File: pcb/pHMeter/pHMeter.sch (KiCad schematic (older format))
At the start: 75 parts, among them J1 Conn_02x03_Odd_Even, J2 Conn_Coaxial_Power, J3 Conn_Coaxial_Power, J4 Conn_Coaxial_Power, J5 RJ12, J6 RJ12, Q1 BSP75, Q2 BSP75, U1 TLV6004PW, U2 TLV6004PW, X1 MINI-USB-SCHIELD-32005-201

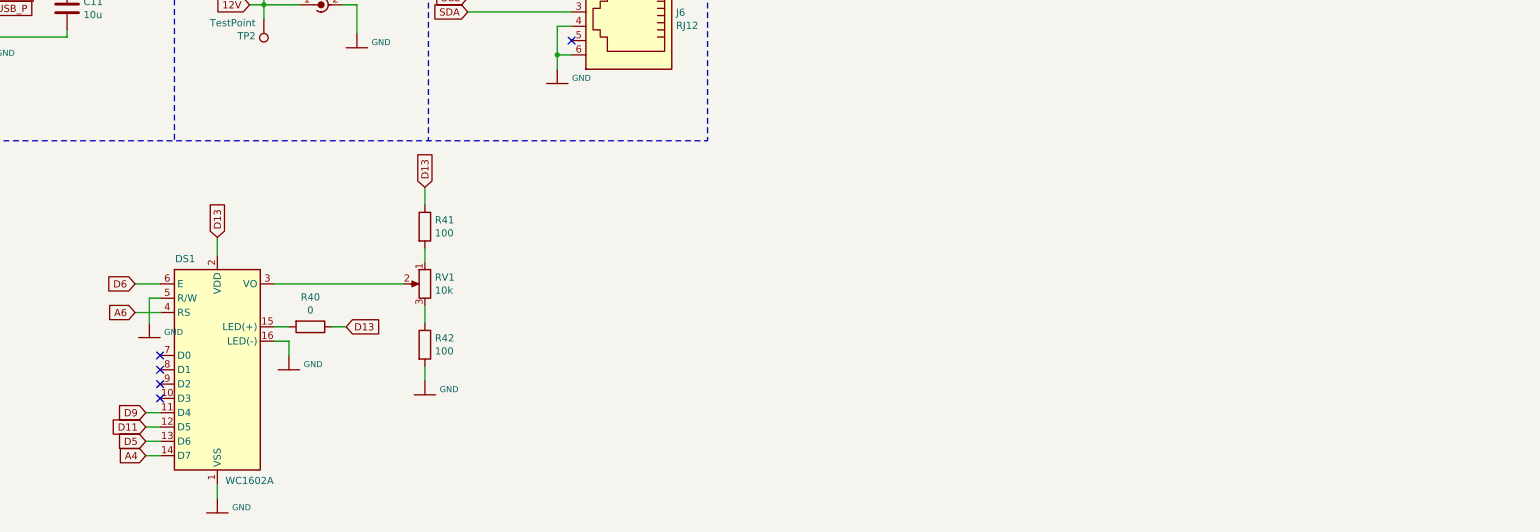
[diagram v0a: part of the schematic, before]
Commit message: change power supply for LCD1602
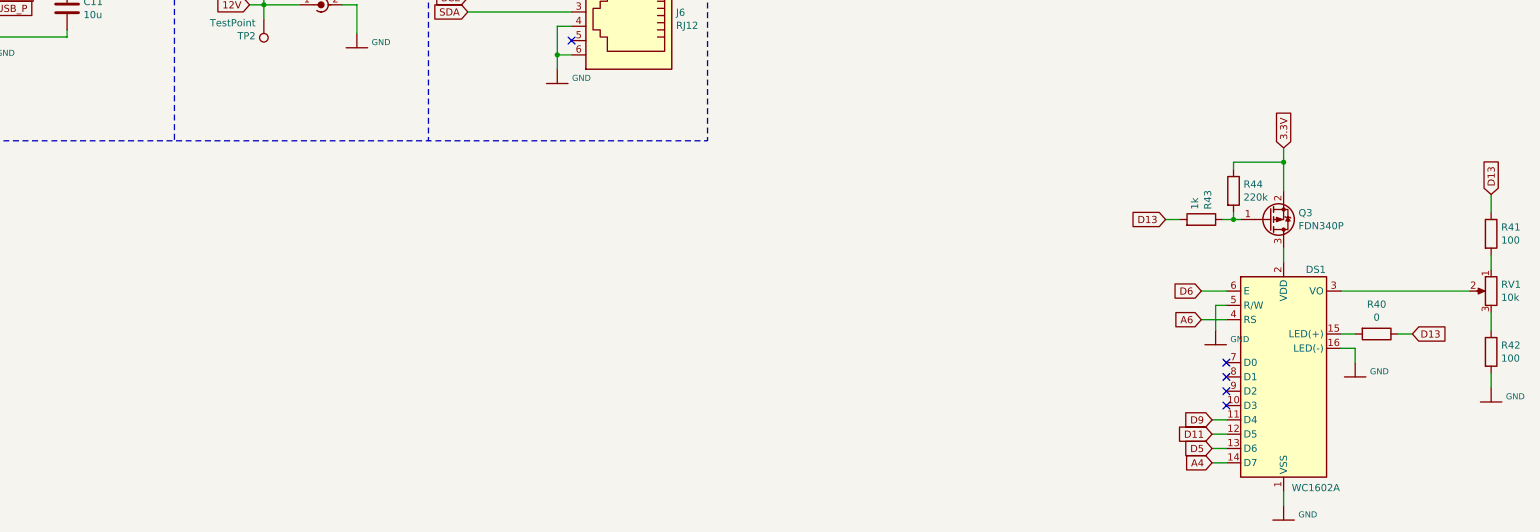
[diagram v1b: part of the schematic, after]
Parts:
- added Q3: FDN340P, Package_TO_SOT_SMD:SOT-23, symbol bioreactor:FDN340P
- added R43: 1k, symbol Device:R
- added R44: 220k, symbol Device:R
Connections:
- net +3V3: now also Q3.2 (S), R44.1
- net D13: now also R43.2; no longer DS1.2 (VDD)
- new net: DS1.2 (VDD), Q3.3 (D)
- new net: Q3.1 (G), R43.1, R44.2
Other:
- moved on the sheet: DS1, R40, R41, R42, RV1
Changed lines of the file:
@@
 	10225 475  10225 7075
+$Comp
+L bioreactor:FDN340P Q3
+U 1 1 5EE2FC2B
+P 14150 7625
+F 0 "Q3" H 14354 7579 50  0000 L CNN
+F 1 "FDN340P" H 14354 7670 50  0000 L CNN
+F 2 "Package_TO_SOT_SMD:SOT-23" H 14350 7550 50  0001 L CIN
+F 3 "https://www.onsemi.com/pub/Collateral/FDN340P-D.PDF" H 14150 7625 50  0001 L CNN
+	1    14150 7625
+	1    0    0    1
+$EndComp
+Wire Wire Line
+	14750 8425 14650 8425
+$Comp
+L Device:R R40
+U 1 1 5EE96652
+P 14900 8425
+F 0 "R40" V 14693 8425 50  0000 C CNN
+F 1 "0" V 14784 8425 50  0000 C CNN
+F 2 "" V 14830 8425 50  0001 C CNN
+F 3 "~" H 14900 8425 50  0001 C CNN
+	1    14900 8425
+	0    1    1    0
+$EndComp
+Wire Wire Line
+	13850 9025 13750 9025
+Wire Wire Line
+	13750 9125 13850 9125
+Wire Wire Line
+	13850 9225 13750 9225
+Wire Wire Line
+	13750 9325 13850 9325
+Text GLabel 13750 9325 0    50   Input ~ 0
+A4
+Text GLabel 13750 9225 0    50   Input ~ 0
+D5
+Text GLabel 13750 9125 0    50   Input ~ 0
+D11
+Text GLabel 13750 9025 0    50   Input ~ 0
+D9
+NoConn ~ 13850 8925
+NoConn ~ 13850 8825
+NoConn ~ 13850 8725
+NoConn ~ 13850 8625
+Wire Wire Line
+	13675 8125 13850 8125
+Text GLabel 13675 8125 0    50   Input ~ 0
+D6
+Wire Wire Line
+	13775 8225 13775 8400
+Wire Wire Line
+	13850 8225 13775 8225
+$Comp
+L Bertha_main-eagle-import:GND #016
+U 1 1 5EF5D01D
+P 13775 8500
+F 0 "#016" H 13825 8550 50  0001 C CNN
+F 1 "GND" H 13878 8538 42  0000 L CNN
+F 2 "" H 13775 8500 50  0001 C CNN
+F 3 "" H 13775 8500 50  0001 C CNN
+	1    13775 8500
+	1    0    0    -1
+$EndComp
+Wire Wire Line
+	13675 8325 13850 8325
+Text GLabel 13675 8325 0    50   Input ~ 0
+A6
+Wire Wire Line
+	15700 7575 15700 7450
+Wire Wire Line
+	15700 7975 15700 7875
+Wire Wire Line
+	15700 8400 15700 8275
+Wire Wire Line
+	15700 8700 15700 8800
+Wire Wire Line
+	15550 8125 14650 8125
+Wire Wire Line
+	15050 8425 15150 8425
+Wire Wire Line
+	14750 8525 14750 8625
+Wire Wire Line
+	14650 8525 14750 8525
+$Comp
+L Bertha_main-eagle-import:GND #018
+U 1 1 5EE96E8F
+P 14750 8725
+F 0 "#018" H 14800 8775 50  0001 C CNN
+F 1 "GND" H 14853 8763 42  0000 L CNN
+F 2 "" H 14750 8725 50  0001 C CNN
+F 3 "" H 14750 8725 50  0001 C CNN
+	1    14750 8725
+	1    0    0    -1
+$EndComp
+Text GLabel 15150 8425 2    50   Input ~ 0
+D13
+$Comp
+L Bertha_main-eagle-import:GND #019
+U 1 1 5EE6ABC2
+P 15700 8900
+F 0 "#019" H 15750 8950 50  0001 C CNN
+F 1 "GND" H 15803 8938 42  0000 L CNN
+F 2 "" H 15700 8900 50  0001 C CNN
+F 3 "" H 15700 8900 50  0001 C CNN
+	1    15700 8900
+	1    0    0    -1
+$EndComp
+$Comp
+L Device:R R42
+U 1 1 5EE6A7EF
+P 15700 8550
+F 0 "R42" H 15770 8596 50  0000 L CNN
+F 1 "100" H 15770 8505 50  0000 L CNN
+F 2 "" V 15630 8550 50  0001 C CNN
+F 3 "~" H 15700 8550 50  0001 C CNN
+	1    15700 8550
+	1    0    0    -1
+$EndComp
+Text GLabel 15700 7450 1    50   Input ~ 0
+D13
+$Comp
+L Device:R R41
+U 1 1 5EE6A2B9
+P 15700 7725
+F 0 "R41" H 15770 7771 50  0000 L CNN
+F 1 "100" H 15770 7680 50  0000 L CNN
+F 2 "" V 15630 7725 50  0001 C CNN
+F 3 "~" H 15700 7725 50  0001 C CNN
+	1    15700 7725
+	1    0    0    -1
+$EndComp
+$Comp
+L Device:R_POT RV1
+U 1 1 5EE688CC
+P 15700 8125
+F 0 "RV1" H 15630 8171 50  0000 R CNN
+F 1 "10k" H 15630 8080 50  0000 R CNN
+F 2 "" H 15700 8125 50  0001 C CNN
+F 3 "~" H 15700 8125 50  0001 C CNN
+	1    15700 8125
+	-1   0    0    -1
+$EndComp
+Text GLabel 13425 7625 0    50   Input ~ 0
+D13
+Wire Wire Line
+	14250 9625 14250 9525
+$Comp
+L Bertha_main-eagle-import:GND #017
+U 1 1 5EE3E294
+P 14250 9725
+F 0 "#017" H 14300 9775 50  0001 C CNN
+F 1 "GND" H 14353 9763 42  0000 L CNN
+F 2 "" H 14250 9725 50  0001 C CNN
+F 3 "" H 14250 9725 50  0001 C CNN
+	1    14250 9725
+	1    0    0    -1
+$EndComp
 $Comp
 L Display_Character:WC1602A DS1
 U 1 1 5EE29EFA
-P 6800 8675
-F 0 "DS1" H 6575 9450 50  0000 C CNN
-F 1 "WC1602A" H 7025 7900 50  0000 C CNN
-F 2 "Display:WC1602A" H 6800 7775 50  0001 C CIN
-F 3 "http://www.wincomlcd.com/pdf/WC1602A-SFYLYHTC06.pdf" H 7500 8675 50  0001 C CNN
-	1    6800 8675
-	1    0    0    -1
-$EndComp
-$Comp
-L Bertha_main-eagle-import:GND #017
-U 1 1 5EE3E294
-P 6800 9675
-F 0 "#017" H 6850 9725 50  0001 C CNN
-F 1 "GND" H 6903 9713 42  0000 L CNN
-F 2 "" H 6800 9675 50  0001 C CNN
-F 3 "" H 6800 9675 50  0001 C CNN
-	1    6800 9675
-	1    0    0    -1
-$EndComp
-Wire Wire Line
-	6800 9575 6800 9475
-Text GLabel 6800 7750 1    50   Input ~ 0
-D13
-Wire Wire Line
-	6800 7750 6800 7875
-$Comp
-L Device:R_POT RV1
-U 1 1 5EE688CC
-P 8250 8075
-F 0 "RV1" H 8180 8121 50  0000 R CNN
-F 1 "10k" H 8180 8030 50  0000 R CNN
-F 2 "" H 8250 8075 50  0001 C CNN
-F 3 "~" H 8250 8075 50  0001 C CNN
-	1    8250 8075
-	-1   0    0    -1
-$EndComp
-$Comp
-L Device:R R41
-U 1 1 5EE6A2B9
-P 8250 7675
-F 0 "R41" H 8320 7721 50  0000 L CNN
-F 1 "100" H 8320 7630 50  0000 L CNN
-F 2 "" V 8180 7675 50  0001 C CNN
-F 3 "~" H 8250 7675 50  0001 C CNN
-	1    8250 7675
-	1    0    0    -1
-$EndComp
-Text GLabel 8250 7400 1    50   Input ~ 0
-D13
-$Comp
-L Device:R R42
-U 1 1 5EE6A7EF
-P 8250 8500
-F 0 "R42" H 8320 8546 50  0000 L CNN
-F 1 "100" H 8320 8455 50  0000 L CNN
-F 2 "" V 8180 8500 50  0001 C CNN
-F 3 "~" H 8250 8500 50  0001 C CNN
-	1    8250 8500
-	1    0    0    -1
-$EndComp
-$Comp
-L Bertha_main-eagle-import:GND #019
-U 1 1 5EE6ABC2
-P 8250 8850
-F 0 "#019" H 8300 8900 50  0001 C CNN
-F 1 "GND" H 8353 8888 42  0000 L CNN
-F 2 "" H 8250 8850 50  0001 C CNN
-F 3 "" H 8250 8850 50  0001 C CNN
-	1    8250 8850
-	1    0    0    -1
-$EndComp
-Text GLabel 7700 8375 2    50   Input ~ 0
-D13
-$Comp
-L Bertha_main-eagle-import:GND #018
-U 1 1 5EE96E8F
-P 7300 8675
-F 0 "#018" H 7350 8725 50  0001 C CNN
-F 1 "GND" H 7403 8713 42  0000 L CNN
-F 2 "" H 7300 8675 50  0001 C CNN
-F 3 "" H 7300 8675 50  0001 C CNN
-	1    7300 8675
-	1    0    0    -1
-$EndComp
-Wire Wire Line
-	7200 8475 7300 8475
-Wire Wire Line
-	7300 8475 7300 8575
-Wire Wire Line
-	7600 8375 7700 8375
-Wire Wire Line
-	8100 8075 7200 8075
-Wire Wire Line
-	8250 8650 8250 8750
-Wire Wire Line
-	8250 8350 8250 8225
-Wire Wire Line
-	8250 7925 8250 7825
-Wire Wire Line
-	8250 7525 8250 7400
-Text GLabel 6225 8275 0    50   Input ~ 0
-A6
-Wire Wire Line
-	6225 8275 6400 8275
-$Comp
-L Bertha_main-eagle-import:GND #016
-U 1 1 5EF5D01D
-P 6325 8450
-F 0 "#016" H 6375 8500 50  0001 C CNN
-F 1 "GND" H 6428 8488 42  0000 L CNN
-F 2 "" H 6325 8450 50  0001 C CNN
-F 3 "" H 6325 8450 50  0001 C CNN
-	1    6325 8450
-	1    0    0    -1
-$EndComp
-Wire Wire Line
-	6400 8175 6325 8175
-Wire Wire Line
-	6325 8175 6325 8350
-Text GLabel 6225 8075 0    50   Input ~ 0
-D6
-Wire Wire Line
-	6225 8075 6400 8075
-NoConn ~ 6400 8575
-NoConn ~ 6400 8675
-NoConn ~ 6400 8775
-NoConn ~ 6400 8875
-Text GLabel 6300 8975 0    50   Input ~ 0
-D9
-Text GLabel 6300 9075 0    50   Input ~ 0
-D11
-Text GLabel 6300 9175 0    50   Input ~ 0
-D5
-Text GLabel 6300 9275 0    50   Input ~ 0
-A4
-Wire Wire Line
-	6300 9275 6400 9275
-Wire Wire Line
-	6400 9175 6300 9175
-Wire Wire Line
-	6300 9075 6400 9075
-Wire Wire Line
-	6400 8975 6300 8975
-$Comp
-L Device:R R40
-U 1 1 5EE96652
-P 7450 8375
-F 0 "R40" V 7243 8375 50  0000 C CNN
-F 1 "0" V 7334 8375 50  0000 C CNN
-F 2 "" V 7380 8375 50  0001 C CNN
-F 3 "~" H 7450 8375 50  0001 C CNN
-	1    7450 8375
-	0    1    1    0
-$EndComp
-Wire Wire Line
-	7300 8375 7200 8375
+P 14250 8725
+F 0 "DS1" H 14475 9475 50  0000 C CNN
+F 1 "WC1602A" H 14475 7950 50  0000 C CNN
+F 2 "Display:WC1602A" H 14250 7825 50  0001 C CIN
+F 3 "http://www.wincomlcd.com/pdf/WC1602A-SFYLYHTC06.pdf" H 14950 8725 50  0001 C CNN
+	1    14250 8725
+	1    0    0    -1
+$EndComp
+$Comp
+L Device:R R44
+U 1 1 5EECAA0A
+P 13900 7425
+F 0 "R44" H 13970 7471 50  0000 L CNN
+F 1 "220k" H 13970 7380 50  0000 L CNN
+F 2 "" V 13830 7425 50  0001 C CNN
+F 3 "~" H 13900 7425 50  0001 C CNN
+	1    13900 7425
+	1    0    0    -1
+$EndComp
+Text GLabel 14250 7125 1    50   Input ~ 0
+3.3V
+Wire Wire Line
+	14250 7125 14250 7225
+$Comp
+L Device:R R43
+U 1 1 5EFDC83F
+P 13675 7625
+F 0 "R43" H 13745 7671 50  0000 L CNN
+F 1 "1k" H 13745 7580 50  0000 L CNN
+F 2 "" V 13605 7625 50  0001 C CNN
+F 3 "~" H 13675 7625 50  0001 C CNN
+	1    13675 7625
+	0    1    -1   0
+$EndComp
+Wire Wire Line
+	13900 7275 13900 7225
+Connection ~ 14250 7225
+Wire Wire Line
+	14250 7225 14250 7425
+Wire Wire Line
+	13900 7225 14250 7225
+Wire Wire Line
+	13900 7575 13900 7625
+Wire Wire Line
+	13900 7625 13950 7625
+Wire Wire Line
+	13825 7625 13900 7625
+Connection ~ 13900 7625
+Wire Wire Line
+	13425 7625 13525 7625
+Wire Wire Line
+	14250 7825 14250 7925
 $EndSCHEMATC
